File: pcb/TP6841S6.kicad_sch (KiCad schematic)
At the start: 9 parts, among them U10 TP6841S6

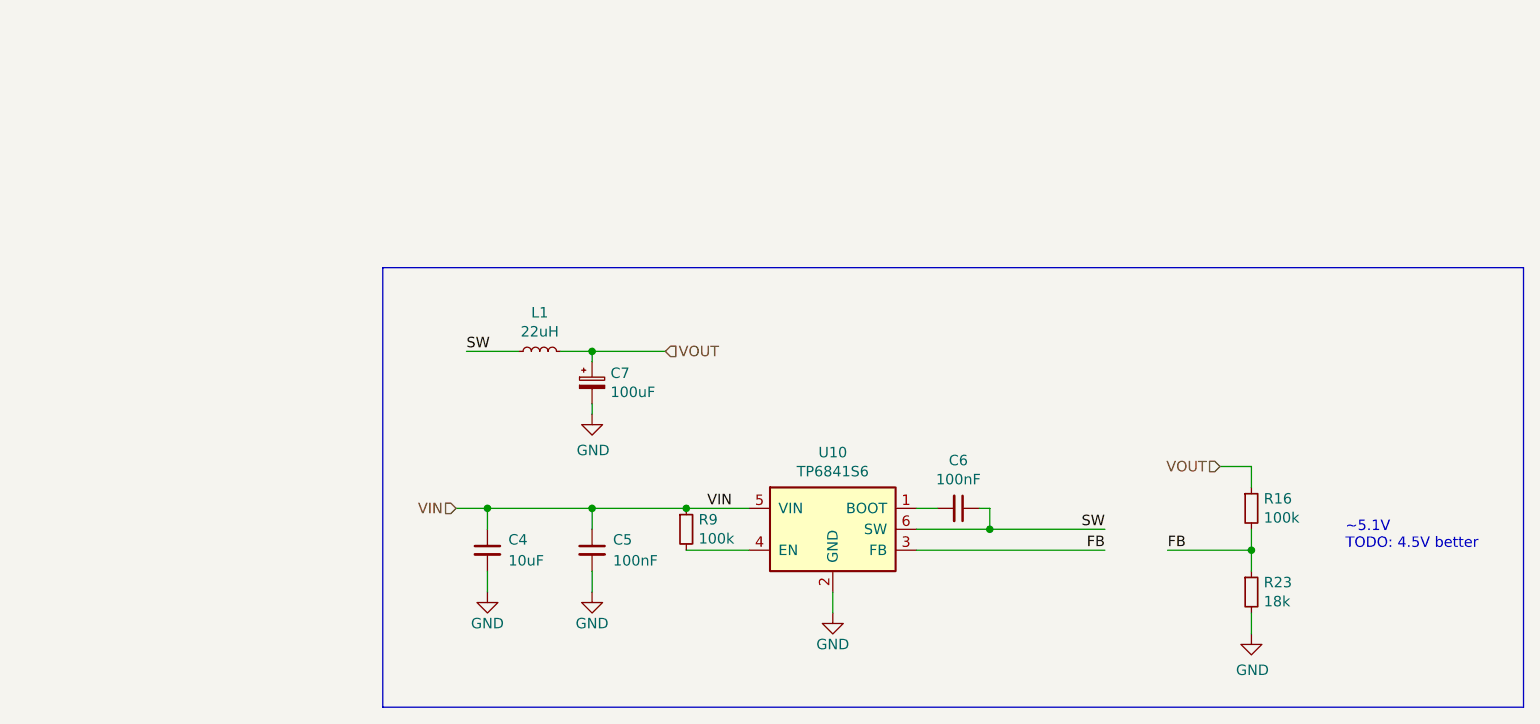
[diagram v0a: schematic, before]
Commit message: Doc files, slight fixes, initial readme.md content
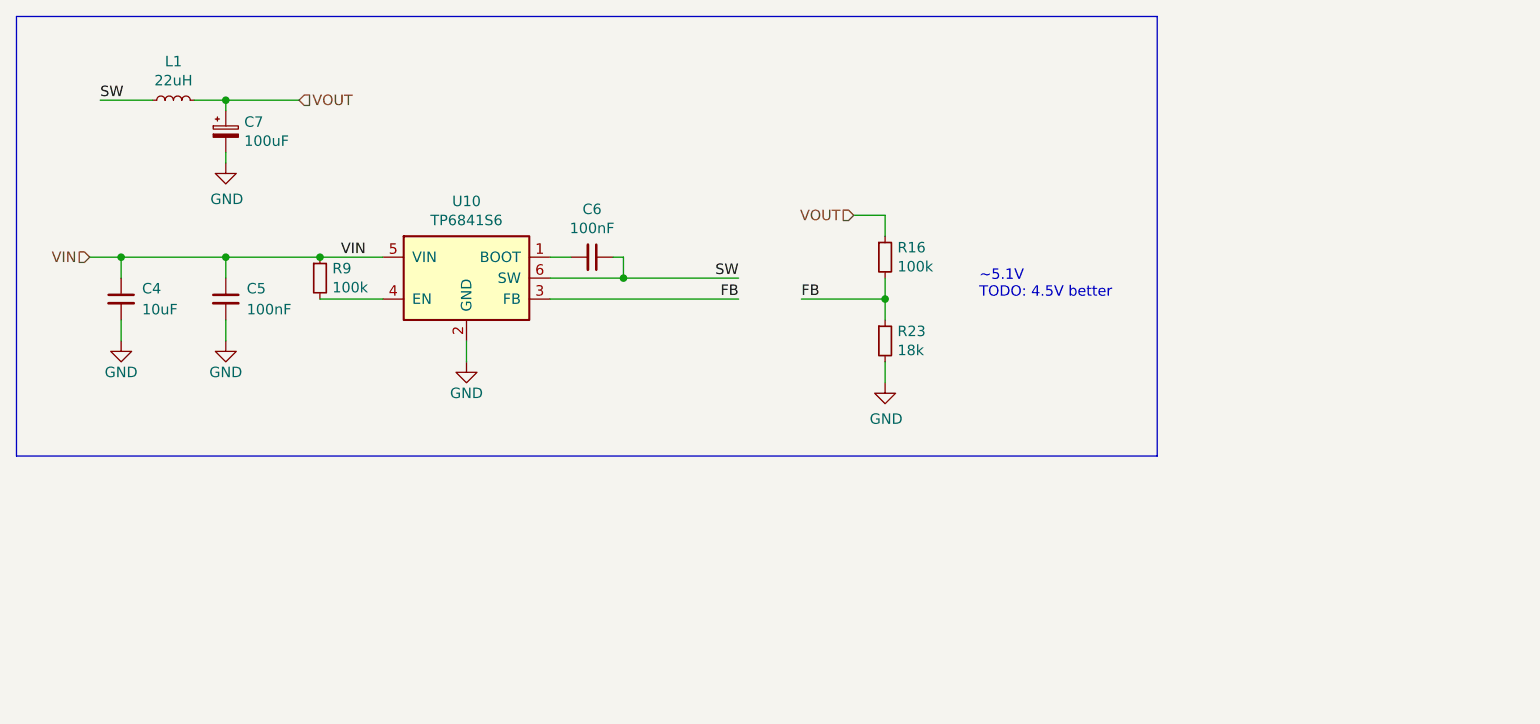
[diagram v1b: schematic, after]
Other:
- moved on the sheet: C4, C5, C6, C7, L1, R16, R23, R9, U10
